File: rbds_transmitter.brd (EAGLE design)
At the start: 160 x 100 mm, 136 parts, among them J2 AVRISP-6, Q1 P-CH, Q2 P-Ch, Q3 P-Ch, T1 ATB3225-75034CT, T2 ATB3225-75034CT, U1 MAX2606, U2 TS974, U3 TS974, U4 MAX1551, U5 ATMEGA328, U6 TPS61030, U7 MCP4812, X1 16Mhz

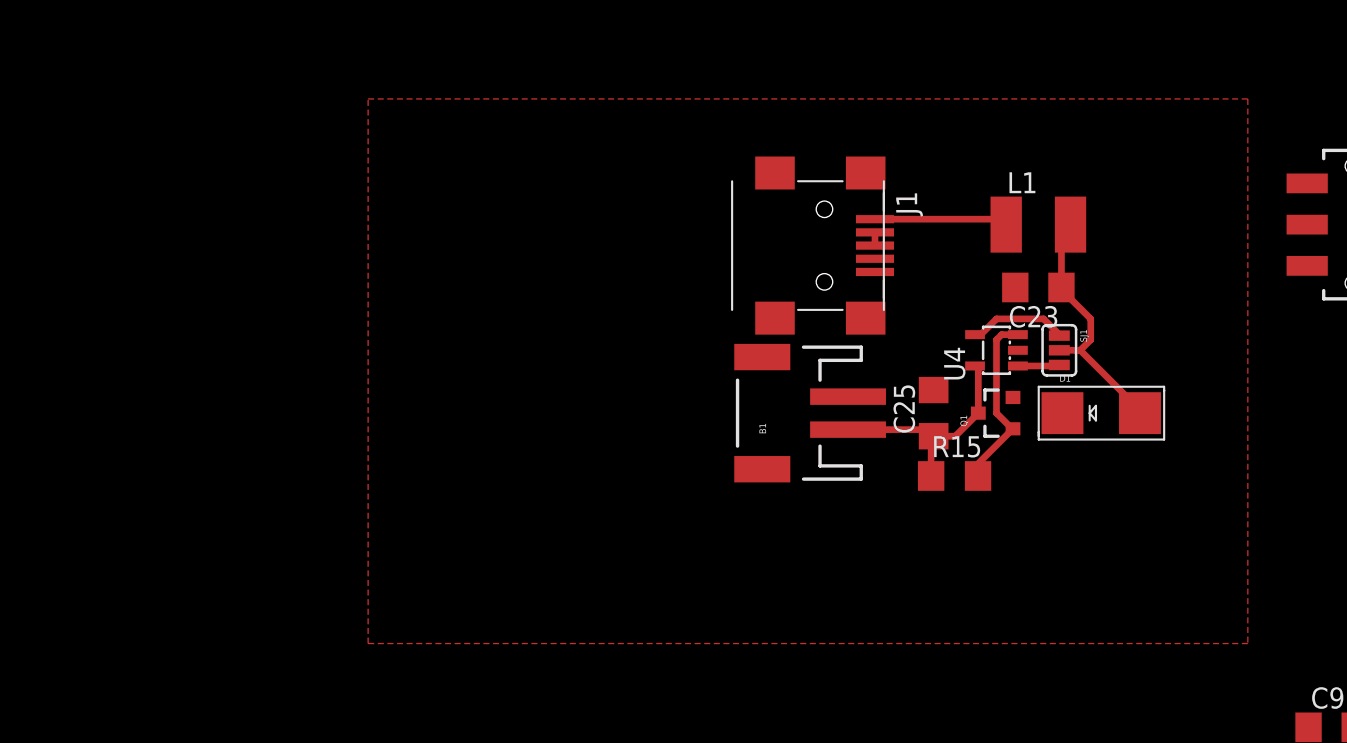
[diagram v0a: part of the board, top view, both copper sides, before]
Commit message: working
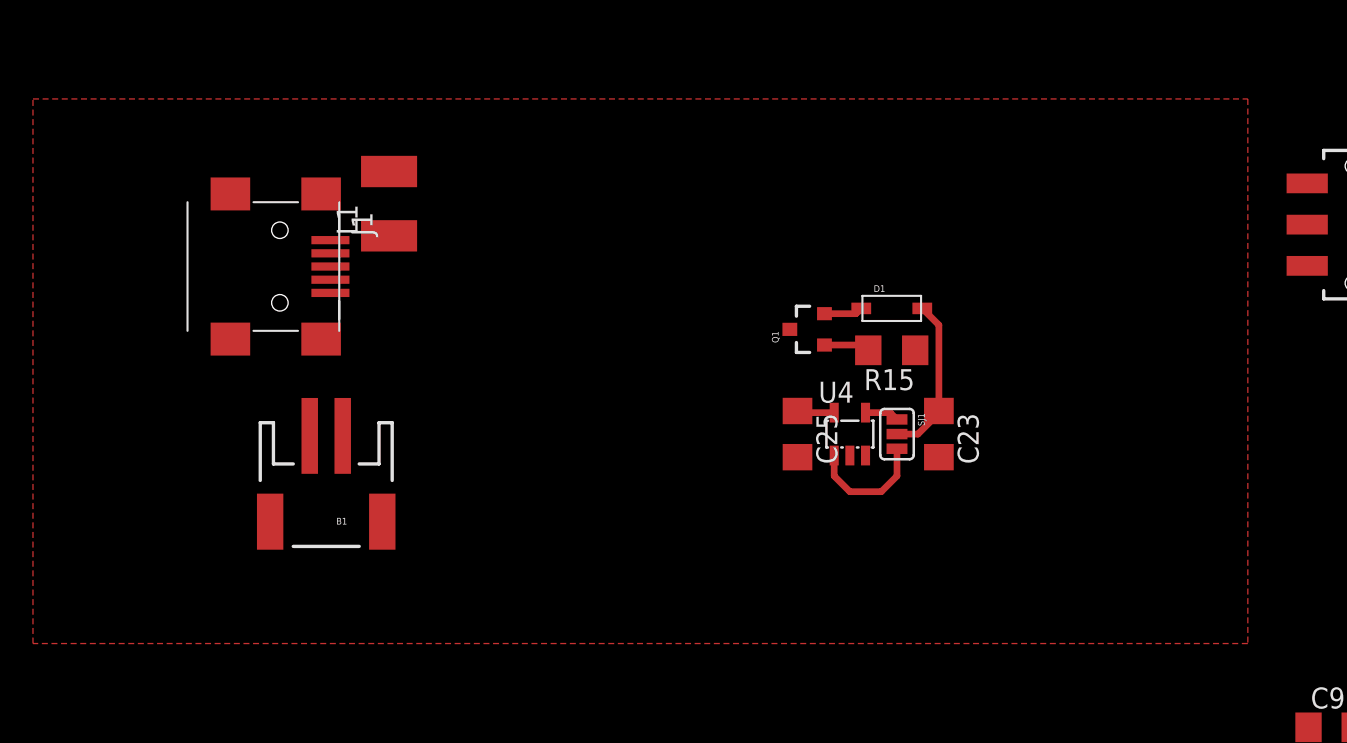
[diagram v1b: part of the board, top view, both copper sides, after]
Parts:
- D1: device adafruit:SMADIODE -> adafruit:SOD-123
- moved L1 39.4 mm to (-163.8, 119.4), turned to 90 degrees
- moved J1 33.0 mm to (-171.4, 115.6)
- moved B1 28.4 mm to (-167.6, 101.6), turned to 180 degrees
- moved D1 14.2 mm to (-133.3, 113.0)
- moved Q1 12.5 mm to (-138.4, 111.8)
- moved SJ1 11.1 mm to (-133.0, 105.4)
- moved C23 10.7 mm to (-130.5, 105.4), turned to 270 degrees
- moved U4 10.2 mm to (-135.9, 105.4), turned to 0 degrees
- moved R15 8.52 mm to (-133.3, 110.5), turned to 180 degrees
- moved C25 8.35 mm to (-139.1, 105.4), turned to 270 degrees
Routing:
- net N$11: track 14.1 -> 2.27 mm
- net N$10: track 11.2 -> 2.79 mm
- net N$54: track 8.09 -> 0.00 mm
- net N$1: track 15.6 -> 9.83 mm
- net N$7: track 2.54 -> 7.49 mm
- net N$8: track 5.96 -> 2.08 mm
- net N$6: track 0.00 -> 2.36 mm
- net N$13: track 0.80 -> 0.00 mm
